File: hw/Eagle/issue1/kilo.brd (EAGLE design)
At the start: 100 x 80 mm, 30 parts, among them IC2 74AC00N, IC3 62256, IC4 74HC138N, Q1 7,3728 MHz

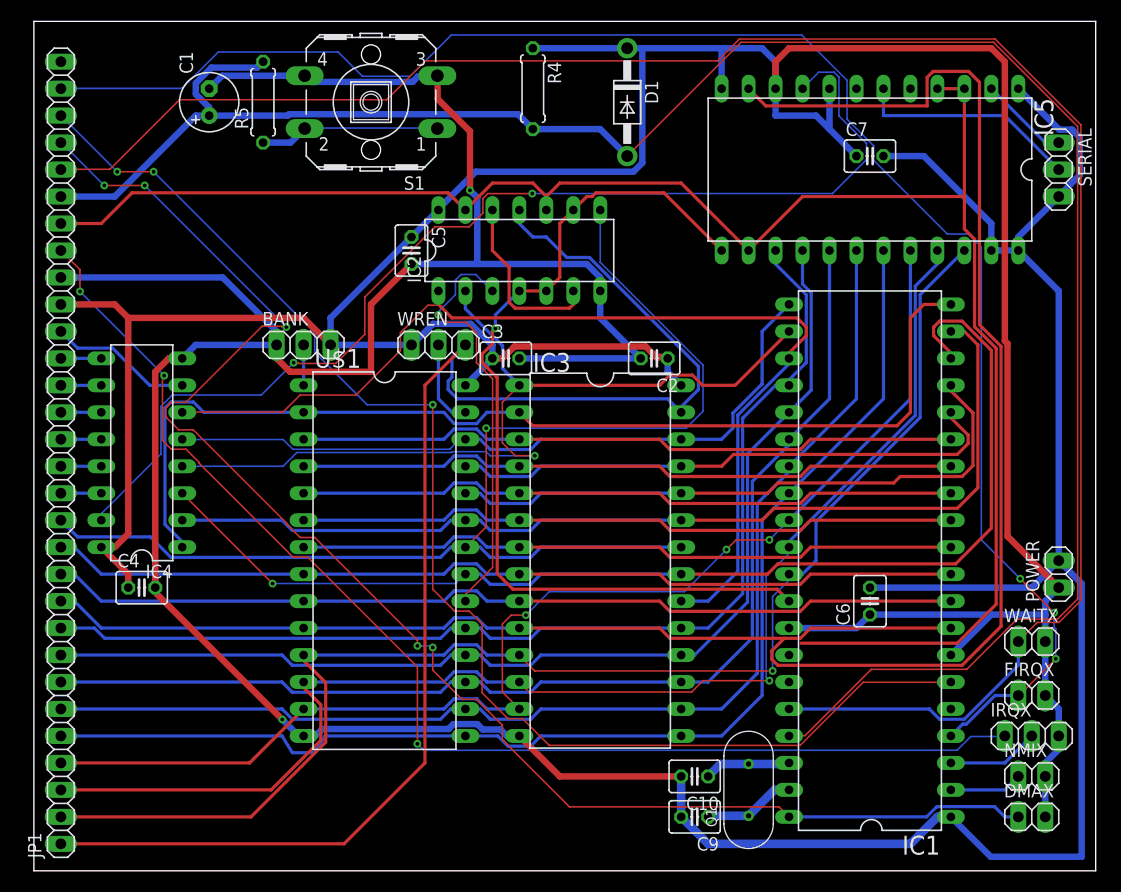
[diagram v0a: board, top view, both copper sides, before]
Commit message: BRD v1 fix
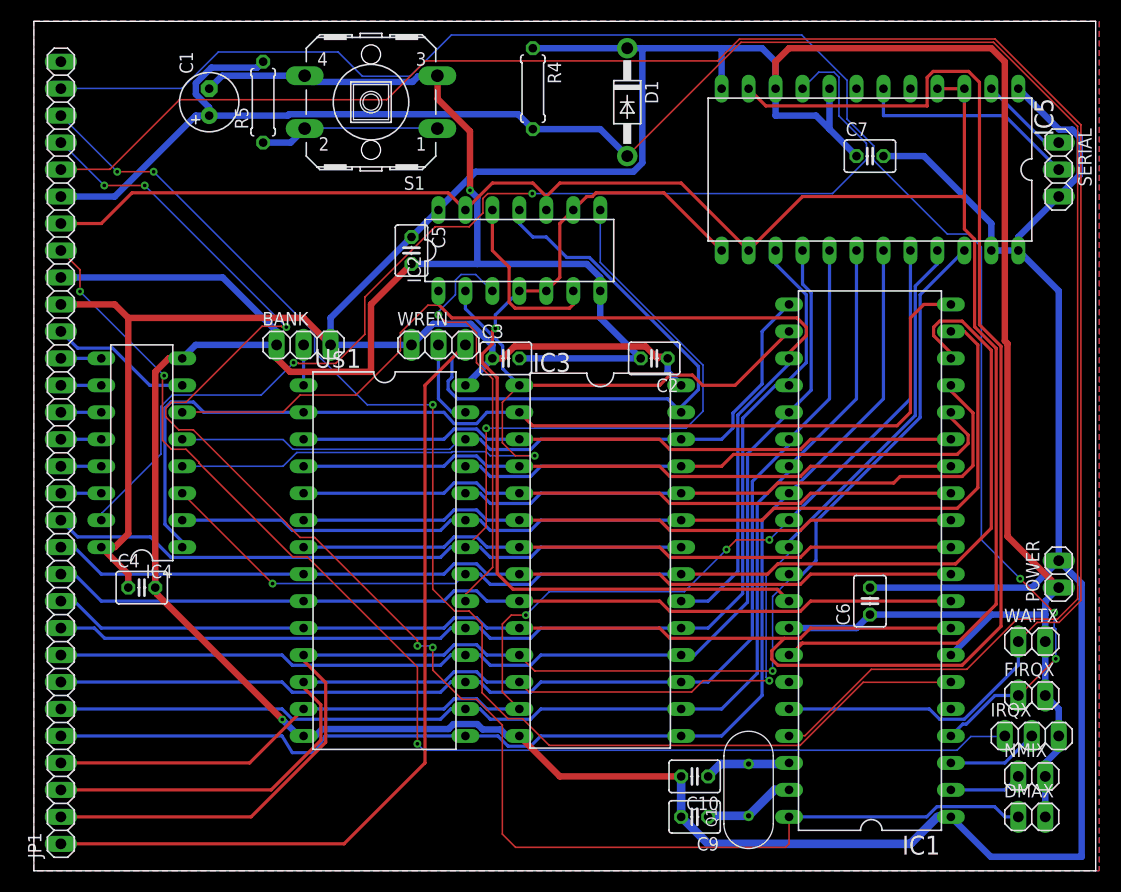
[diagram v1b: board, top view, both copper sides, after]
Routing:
- net /BUSRQ: track 142.9 -> 152.0 mm
- net E: track 166.0 -> 167.8 mm
- added copper zone on layer 1, net +5V
- added copper zone on layer 16, net GND
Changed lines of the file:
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@@
 <via x="41.0718" y="64.0842" extent="1-16" drill="0.35"/>
 <via x="23.3934" y="14.2494" extent="1-16" drill="0.35"/>
+<polygon width="0.3048" layer="16">
+<vertex x="0" y="80.01"/>
+<vertex x="100.33" y="80.01"/>
+<vertex x="100.33" y="0"/>
+<vertex x="0" y="0"/>
+</polygon>
 </signal>
 <signal name="PHI0">
@@
 <wire x1="59.534734375" y1="48.415265625" x2="59.69" y2="48.26" width="0.6096" layer="1"/>
 <wire x1="59.69" y1="48.26" x2="59.69" y2="46.99" width="0.6096" layer="16"/>
+<polygon width="0.3048" layer="1">
+<vertex x="0" y="80.01"/>
+<vertex x="100.33" y="80.01"/>
+<vertex x="100.33" y="0"/>
+<vertex x="0" y="0"/>
+</polygon>
 </signal>
 <signal name="A0">
@@
 <wire x1="41.6814" y1="16.1544" x2="40.3098" y2="16.1544" width="0.1524" layer="1"/>
 <wire x1="44.1198" y1="13.716" x2="41.6814" y2="16.1544" width="0.1524" layer="1"/>
-<wire x1="44.1198" y1="12.3444" x2="44.1198" y2="13.716" width="0.1524" layer="1"/>
-<wire x1="50.4444" y1="6.0198" x2="44.1198" y2="12.3444" width="0.1524" layer="1"/>
-<wire x1="70.1802" y1="6.0198" x2="50.4444" y2="6.0198" width="0.1524" layer="1"/>
-<wire x1="71.12" y1="5.08" x2="70.1802" y2="6.0198" width="0.1524" layer="1"/>
+<wire x1="44.1198" y1="3.4544" x2="44.1198" y2="13.716" width="0.1524" layer="1"/>
+<wire x1="45.3644" y1="2.2098" x2="44.1198" y2="3.4544" width="0.1524" layer="1"/>
+<wire x1="70.7898" y1="2.2098" x2="45.3644" y2="2.2098" width="0.1524" layer="1"/>
 <wire x1="2.5908" y1="68.58" x2="2.54" y2="68.58" width="0.1524" layer="16"/>
 <via x="6.6294" y="64.5414" extent="1-16" drill="0.35"/>
@@
 <via x="36.1188" y="21.1836" extent="1-16" drill="0.35"/>
 <via x="37.5666" y="21.0312" extent="1-16" drill="0.35"/>
+<wire x1="71.12" y1="2.54" x2="70.7898" y2="2.2098" width="0.1524" layer="1"/>
+<wire x1="71.12" y1="5.08" x2="71.12" y2="2.54" width="0.1524" layer="1"/>
 </signal>
 <signal name="/BUSACK">
@@
 <wire x1="87.63" y1="63.5" x2="87.63" y2="73.66" width="0.3048" layer="1"/>
 <wire x1="88.5952" y1="59.4802" x2="87.63" y2="60.4454" width="0.3048" layer="1"/>
-<wire x1="72.2376" y1="21.4376" x2="86.963" y2="21.4376" width="0.3048" layer="1"/>
+<wire x1="72.2376" y1="21.4376" x2="72.39" y2="21.4376" width="0.3048" layer="1"/>
+<wire x1="72.39" y1="21.4376" x2="86.963" y2="21.4376" width="0.3048" layer="1"/>
 <wire x1="90.6272" y1="49.20478125" x2="88.5952" y2="51.23678125" width="0.3048" layer="1"/>
 <wire x1="88.5952" y1="51.23678125" x2="88.5952" y2="59.4802" width="0.3048" layer="1"/>
@@
 <wire x1="43.18" y1="64.77" x2="40.64" y2="62.23" width="0.3048" layer="1"/>
 <wire x1="40.64" y1="62.23" x2="39.0144" y2="63.8556" width="0.3048" layer="1"/>
+<wire x1="71.12" y1="20.32" x2="71.2724" y2="20.32" width="0.3048" layer="1"/>
+<wire x1="71.2724" y1="20.32" x2="72.39" y2="21.4376" width="0.3048" layer="1"/>
 <wire x1="48.26" y1="63.5" x2="48.26" y2="62.23" width="0" layer="19" extent="1-1"/>
-<wire x1="71.12" y1="20.32" x2="72.2376" y2="21.4376" width="0" layer="19" extent="1-1"/>
 </signal>
 </signals>
